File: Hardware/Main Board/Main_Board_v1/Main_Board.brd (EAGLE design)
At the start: 160 x 108.9 mm, 59 parts, among them IC1 MBED_MICROCONTROLLER, IC2 LM311N, IC3 MCP602P, IC4 MCP602P, IC5 4072N, Q1 IRF3704, Q2 BS170

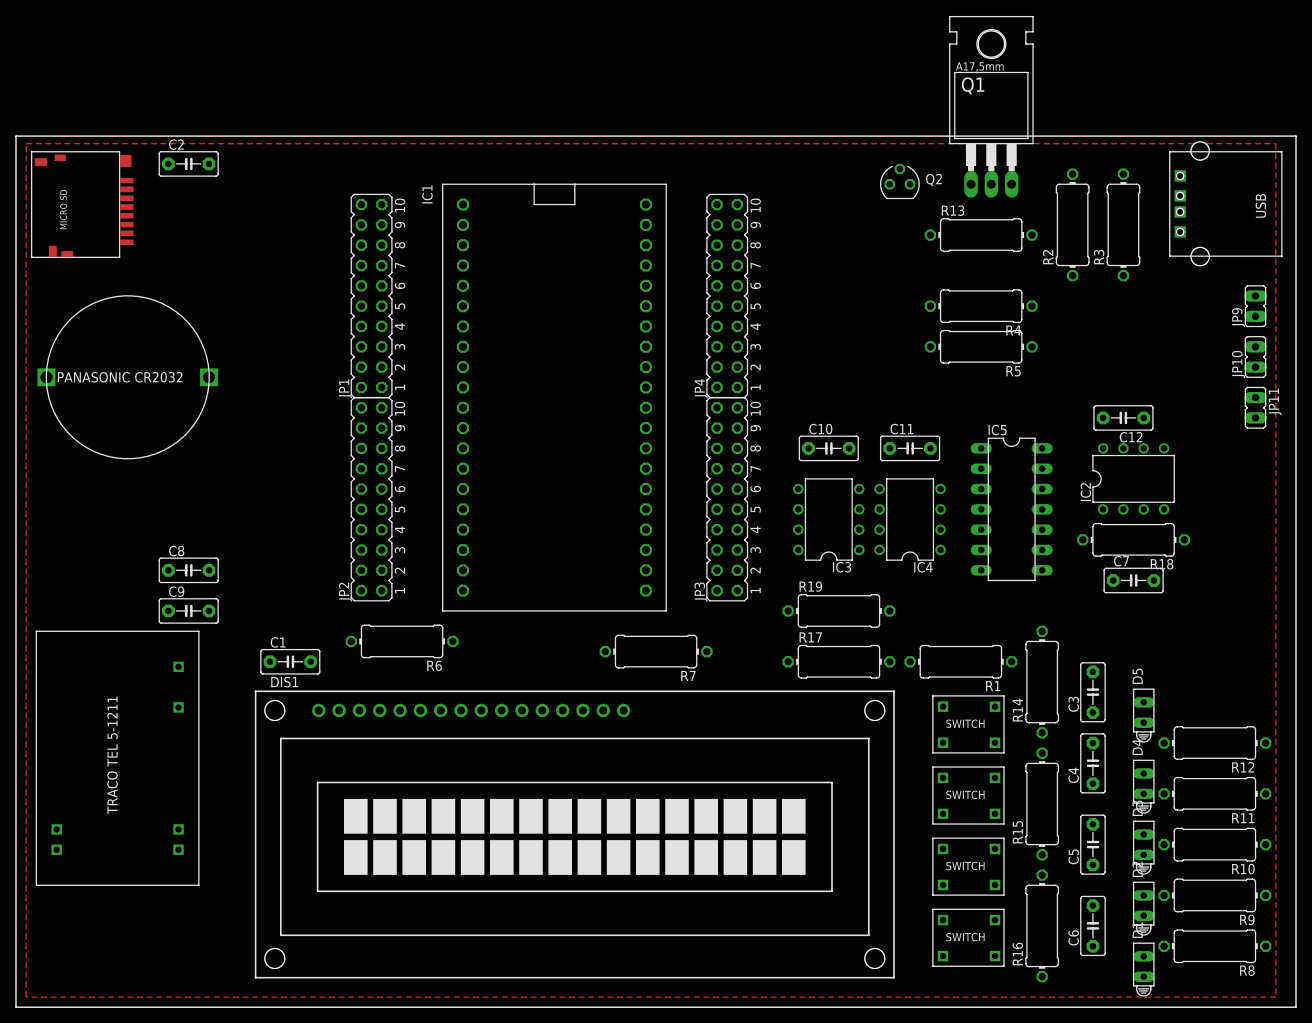
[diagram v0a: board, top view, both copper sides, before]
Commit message: Main Board Work in Progress
Work in Progress on the main board.
Need to test the timing circuit and then finalize and finish routing the
board.
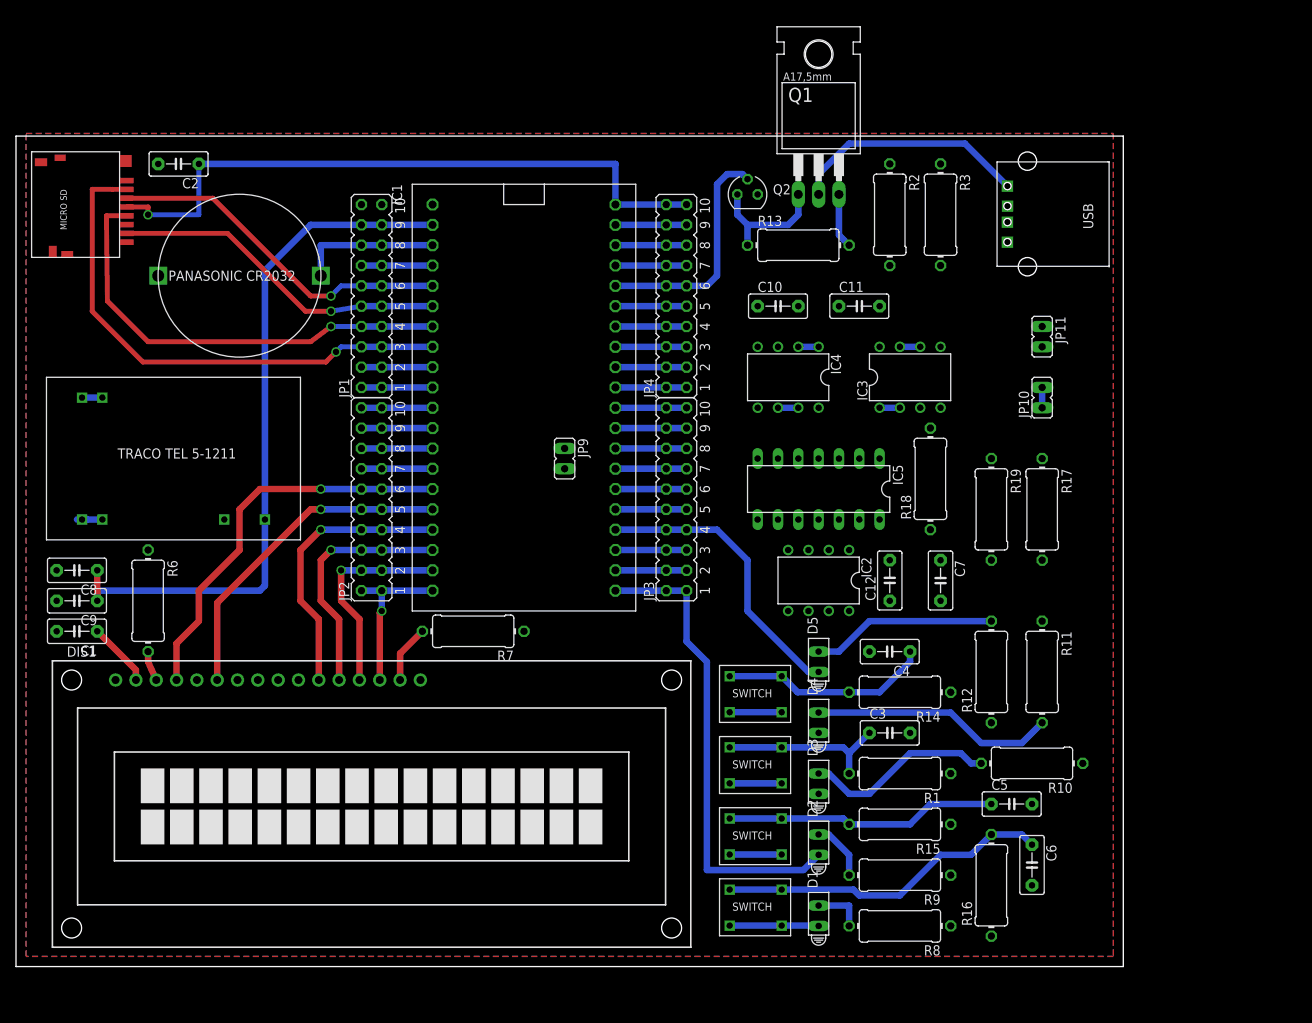
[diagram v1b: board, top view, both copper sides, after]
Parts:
- removed R4, R5: (no value), rcl:0411/12
- moved JP9 88.4 mm to (69.8, 67.3), turned to 180 degrees
- moved POWER_SUPPLY 43.8 mm to (8.89, 59.7), turned to 0 degrees
- moved IC2 41.4 mm to (101.6, 52.1), turned to 180 degrees
- moved D2 41.3 mm to (101.6, 19.1)
- moved D3 41.3 mm to (101.6, 26.7)
- moved D4 41.3 mm to (101.6, 34.3)
- moved D1 41.1 mm to (101.6, 10.2)
- moved D5 41.1 mm to (101.6, 41.9)
- moved R8 39.5 mm to (111.8, 8.89)
- moved R9 39.5 mm to (111.8, 15.2)
- moved C12 35.6 mm to (110.5, 52.1), turned to 90 degrees
- moved R6 32.2 mm to (17.8, 49.5), turned to 270 degrees
- moved R17 31.7 mm to (129.5, 61.0), turned to 270 degrees
- moved R12 29.3 mm to (123.2, 40.6), turned to 90 degrees
- moved C4 29.0 mm to (110.5, 43.2), turned to 180 degrees
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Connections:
- net 5V_MBED: no longer R4.2, R5.2
- net P30: now also C6.1, IC4.5, R16.2, U$8.1, U$8.2; no longer Q2.G
- net P36: now also Q2.G; no longer C6.1, IC4.5, R16.2, U$8.1, U$8.2
- net SCL: no longer R5.1
- net SDA: no longer R4.1
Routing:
- net VIN: track 0.00 -> 89.0 mm
- net 3V3_MBED: track 0.00 -> 82.4 mm, vias 0 -> 1
- net P8: track 0.00 -> 65.5 mm, vias 0 -> 1
- net P21: track 0.00 -> 59.6 mm
- net P7: track 0.00 -> 56.6 mm, vias 0 -> 1
- net P30: track 0.00 -> 50.7 mm
- net 5V_MBED: track 0.00 -> 50.2 mm
- net P15: track 0.00 -> 49.8 mm, vias 0 -> 1
- net P5: track 0.00 -> 43.8 mm, vias 0 -> 1
- net P35: track 0.00 -> 43.0 mm
- net P6: track 0.00 -> 42.3 mm, vias 0 -> 1
- net P16: track 0.00 -> 41.4 mm, vias 0 -> 1
- net P24: track 0.00 -> 36.5 mm
- net P34: track 0.00 -> 35.3 mm
- net P17: track 0.00 -> 34.8 mm, vias 0 -> 1
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- added copper zone on layer 16, net GND
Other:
- board size 160 x 108.9 mm -> 138.4 x 103.8 mm
